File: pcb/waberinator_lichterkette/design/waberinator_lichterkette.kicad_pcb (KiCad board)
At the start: 2 copper layers, 25.8 x 10.3 mm, 9 parts

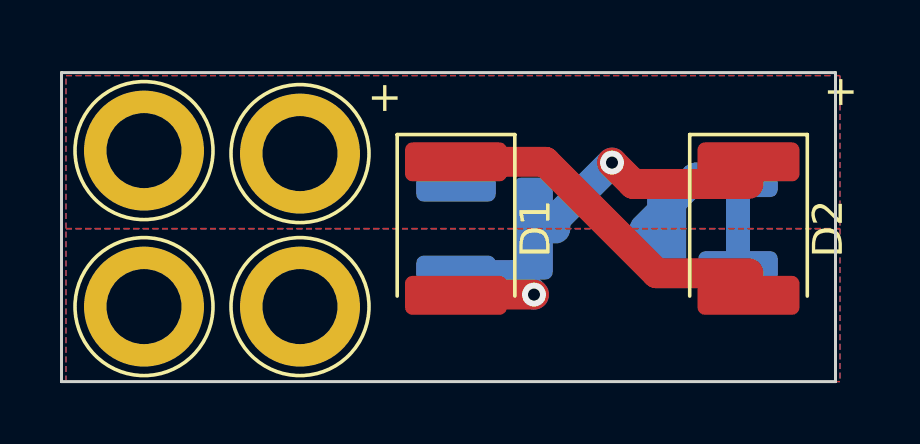
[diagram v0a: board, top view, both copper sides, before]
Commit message: [HW] finish layout
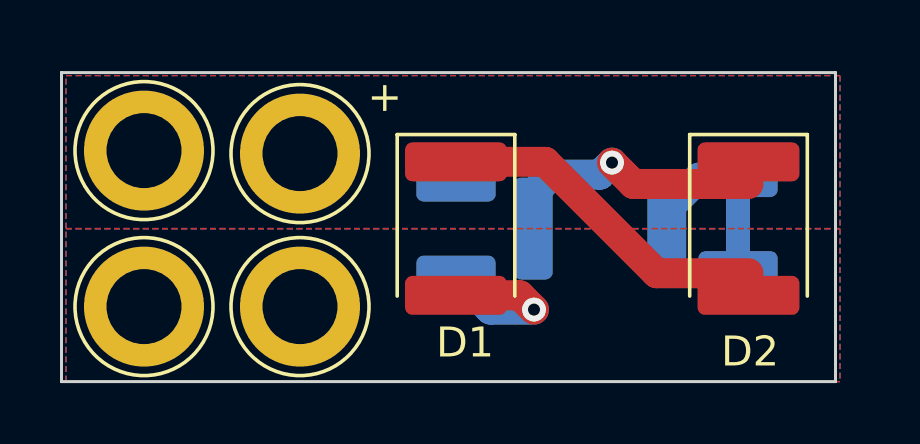
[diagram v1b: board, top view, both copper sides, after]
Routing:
- net Net-(D2-K): track 7.83 -> 9.07 mm
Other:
- board text added: "Lichterkette v11"
- board text removed: "Lichterkette v10"
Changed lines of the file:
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@@
     (property "ki_keywords" "LED diode")
     (attr smd)
-    (fp_text reference "D2" (at 0 -2.65 -90) (layer "F.SilkS")
+    (fp_text reference "D2" (at 4.1 -0.05) (layer "F.SilkS")
         (effects (font (size 1 1) (thickness 0.15)))
     )
@@
     (fp_line (start 2.25 1.6) (end 2.25 -1.6)
       (stroke (width 0.1) (type solid)) (layer "F.Fab"))
-    (pad "1" smd roundrect (at -2.225 0 270) (size 1.3 3.4) (layers "F.Cu" "F.Paste" "F.Mask") (roundrect_rratio 0.192308)
+    (pad "1" smd roundrect (at -2.225 0 270) (size 1.3 3.4) (layers "F.Cu" "F.Paste" "F.Mask") (roundrect_rratio 0.1923076923)
       (net 3 "Net-(D2-K)") (pinfunction "K") (pintype "passive"))
-    (pad "2" smd roundrect (at 2.225 0 270) (size 1.3 3.4) (layers "F.Cu" "F.Paste" "F.Mask") (roundrect_rratio 0.192308)
+    (pad "2" smd roundrect (at 2.225 0 270) (size 1.3 3.4) (layers "F.Cu" "F.Paste" "F.Mask") (roundrect_rratio 0.1923076923)
       (net 1 "Net-(D1-K)") (pinfunction "A") (pintype "passive"))
     (model "${KICAD6_3DMODEL_DIR}/LED_SMD.3dshapes/LED_1812_4532Metric.wrl"
@@
     (property "ki_keywords" "LED diode")
     (attr smd)
-    (fp_text reference "D1" (at 0 -2.65 -90) (layer "F.SilkS")
+    (fp_text reference "D1" (at 3.8 -0.3) (layer "F.SilkS")
         (effects (font (size 1 1) (thickness 0.15)))
     )
@@
     (property "ki_keywords" "R res resistor")
     (attr smd)
-    (fp_text reference "R1" (at -3.6 0 -180) (layer "B.SilkS")
+    (fp_text reference "R1" (at -3.8 0.1 -180) (layer "B.SilkS")
         (effects (font (size 1 1) (thickness 0.15)) (justify mirror))
     )
@@
     (property "ki_keywords" "LED diode")
     (attr smd)
-    (fp_text reference "D3" (at 0 2.65) (layer "B.SilkS")
+    (fp_text reference "D3" (at 0 3.4) (layer "B.SilkS")
         (effects (font (size 1 1) (thickness 0.15)) (justify mirror))
     )
@@
     (fp_line (start 2.25 1.6) (end -1.45 1.6)
       (stroke (width 0.1) (type solid)) (layer "B.Fab"))
-    (pad "1" smd roundrect (at -2.225 0 180) (size 1.3 3.4) (layers "B.Cu" "B.Paste" "B.Mask") (roundrect_rratio 0.192308)
+    (pad "1" smd roundrect (at -2.225 0 180) (size 1.3 3.4) (layers "B.Cu" "B.Paste" "B.Mask") (roundrect_rratio 0.1923076923)
       (net 4 "Net-(D3-K)") (pinfunction "K") (pintype "passive"))
-    (pad "2" smd roundrect (at 2.225 0 180) (size 1.3 3.4) (layers "B.Cu" "B.Paste" "B.Mask") (roundrect_rratio 0.192308)
+    (pad "2" smd roundrect (at 2.225 0 180) (size 1.3 3.4) (layers "B.Cu" "B.Paste" "B.Mask") (roundrect_rratio 0.1923076923)
       (net 3 "Net-(D2-K)") (pinfunction "A") (pintype "passive"))
     (model "${KICAD6_3DMODEL_DIR}/LED_SMD.3dshapes/LED_1812_4532Metric.wrl"
@@
     (property "ki_keywords" "R res resistor")
     (attr smd)
-    (fp_text reference "R2" (at -3.45 0 -180) (layer "B.SilkS")
+    (fp_text reference "R2" (at -3.75 -0.2 -180) (layer "B.SilkS")
         (effects (font (size 1 1) (thickness 0.15)) (justify mirror))
     )
@@
     )
   )
-  (gr_line (start 140.4 77.6) (end 140.4 80.6)
+  (gr_line (start 140.4 77.55) (end 140.4 80.55)
     (stroke (width 0.8) (type default)) (layer "B.Cu"))
   (gr_line (start 121.45 79.25) (end 153.3 79.25)
@@
     (effects (font (size 1 1) (thickness 0.15)) (justify left bottom mirror))
   )
-  (gr_text "+" (at 144.4 75.2) (layer "B.SilkS")
-    (effects (font (size 1 1) (thickness 0.15)) (justify left bottom mirror))
-  )
   (gr_text "+" (at 129.2 75.4) (layer "F.SilkS")
     (effects (font (size 1 1) (thickness 0.15)) (justify left bottom mirror))
   )
-  (gr_text "+" (at 144.4 75.2) (layer "F.SilkS")
-    (effects (font (size 1 1) (thickness 0.15)) (justify left bottom mirror))
-  )
   (gr_text "+" (at 129.8 75.4) (layer "B.Mask")
     (effects (font (size 1 1) (thickness 0.15)) (justify left bottom mirror))
   )
-  (gr_text "Lichterkette v10" (at 141.8 83.8) (layer "B.Mask")
+  (gr_text "Lichterkette v11" (at 141.8 83.8) (layer "B.Mask")
     (effects (font (size 1 1) (thickness 0.15)) (justify left bottom mirror))
   )
@@
   (segment (start 133.975 76.975) (end 137.6875 80.6875) (width 1) (layer "F.Cu") (net 1))
   (segment (start 133.975 76.975) (end 131 76.975) (width 1) (layer "F.Cu") (net 1))
-  (segment (start 131.025 81.4) (end 131 81.425) (width 1) (layer "F.Cu") (net 2))
-  (segment (start 133.6 81.4) (end 131.025 81.4) (width 1) (layer "F.Cu") (net 2))
-  (via (at 133.6 81.4) (size 0.8) (drill 0.4) (layers "F.Cu" "B.Cu") (net 2))
-  (segment (start 133.6 81.4) (end 132.95 80.75) (width 1) (layer "B.Cu") (net 2))
-  (segment (start 132.95 80.75) (end 131 80.75) (width 1) (layer "B.Cu") (net 2))
+  (segment (start 133.6 81.9) (end 133.125 81.425) (width 1) (layer "F.Cu") (net 2))
+  (segment (start 133.125 81.425) (end 131 81.425) (width 1) (layer "F.Cu") (net 2))
+  (via (at 133.6 81.9) (size 0.8) (drill 0.4) (layers "F.Cu" "B.Cu") (net 2))
+  (segment (start 132.15 81.9) (end 131 80.75) (width 1) (layer "B.Cu") (net 2))
+  (segment (start 133.6 81.9) (end 132.15 81.9) (width 1) (layer "B.Cu") (net 2))
   (segment (start 136.9125 77.7125) (end 140.75 77.7125) (width 1) (layer "F.Cu") (net 3))
   (segment (start 136.2 77) (end 136.9125 77.7125) (width 1) (layer "F.Cu") (net 3))
   (via (at 136.2 77) (size 0.8) (drill 0.4) (layers "F.Cu" "B.Cu") (net 3))
-  (segment (start 136.2 77) (end 134.3125 78.8875) (width 1) (layer "B.Cu") (net 3))
-  (segment (start 134.3125 78.8875) (end 134.3125 79.2) (width 1) (layer "B.Cu") (net 3))
-  (segment (start 137.2875 79.2) (end 138.9875 77.5) (width 1) (layer "B.Cu") (net 4))
-  (segment (start 138.9875 77.5) (end 140.4 77.5) (width 1) (layer "B.Cu") (net 4))
+  (segment (start 133.575 78.025) (end 134.2 77.4) (width 1) (layer "B.Cu") (net 3))
+  (segment (start 135.8 77.4) (end 136.2 77) (width 1) (layer "B.Cu") (net 3))
+  (segment (start 134.2 77.4) (end 135.8 77.4) (width 1) (layer "B.Cu") (net 3))
+  (segment (start 133.575 79.2) (end 133.575 78.025) (width 1) (layer "B.Cu") (net 3))
+  (segment (start 138.025 78.575) (end 138.025 79.2) (width 1) (layer "B.Cu") (net 4))
+  (segment (start 139.1 77.5) (end 138.025 78.575) (width 1) (layer "B.Cu") (net 4))
+  (segment (start 140.4 77.5) (end 139.1 77.5) (width 1) (layer "B.Cu") (net 4))
   (zone (net 5) (net_name "Net-(R1-Pad1)") (layers "F&B.Cu") (hatch edge 0.5)
     (priority 1)
@@
   )
   (zone (net 6) (net_name "Net-(R2-Pad2)") (layers "F&B.Cu") (hatch edge 0.5)
-    (connect_pads (clearance 0.5))
+    (connect_pads (clearance 0.25))
     (min_thickness 0.25) (filled_areas_thickness no)
-    (fill yes (thermal_gap 0.5) (thermal_bridge_width 0.5))
+    (fill yes (thermal_gap 0.2) (thermal_bridge_width 0.5))
     (polygon
       (pts
